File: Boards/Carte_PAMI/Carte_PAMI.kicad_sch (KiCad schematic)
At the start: 41 parts, among them J1 Emergency BTN, J10 DC Motor B, J2 USB_C_Receptacle_USB2.0_16P, J3 VL53L0X_1, J4 VL53L0X_2, J5 Battery_connector, J6 ELRS_Module, J7 Tirette, J8 DC Motor A, J9 Odom_Shield, Q1 PMOS, SW1 SW_Push, SW2 SW_Push, SW3 SW_Nidec_CAS-120A1, U1 ESP32-S3-WROOM-1U-N16R8, U2 USBLC6-2SC6, U3 TLV76150DCY, U4 TLV76133DCY, U5 TB6612FNG

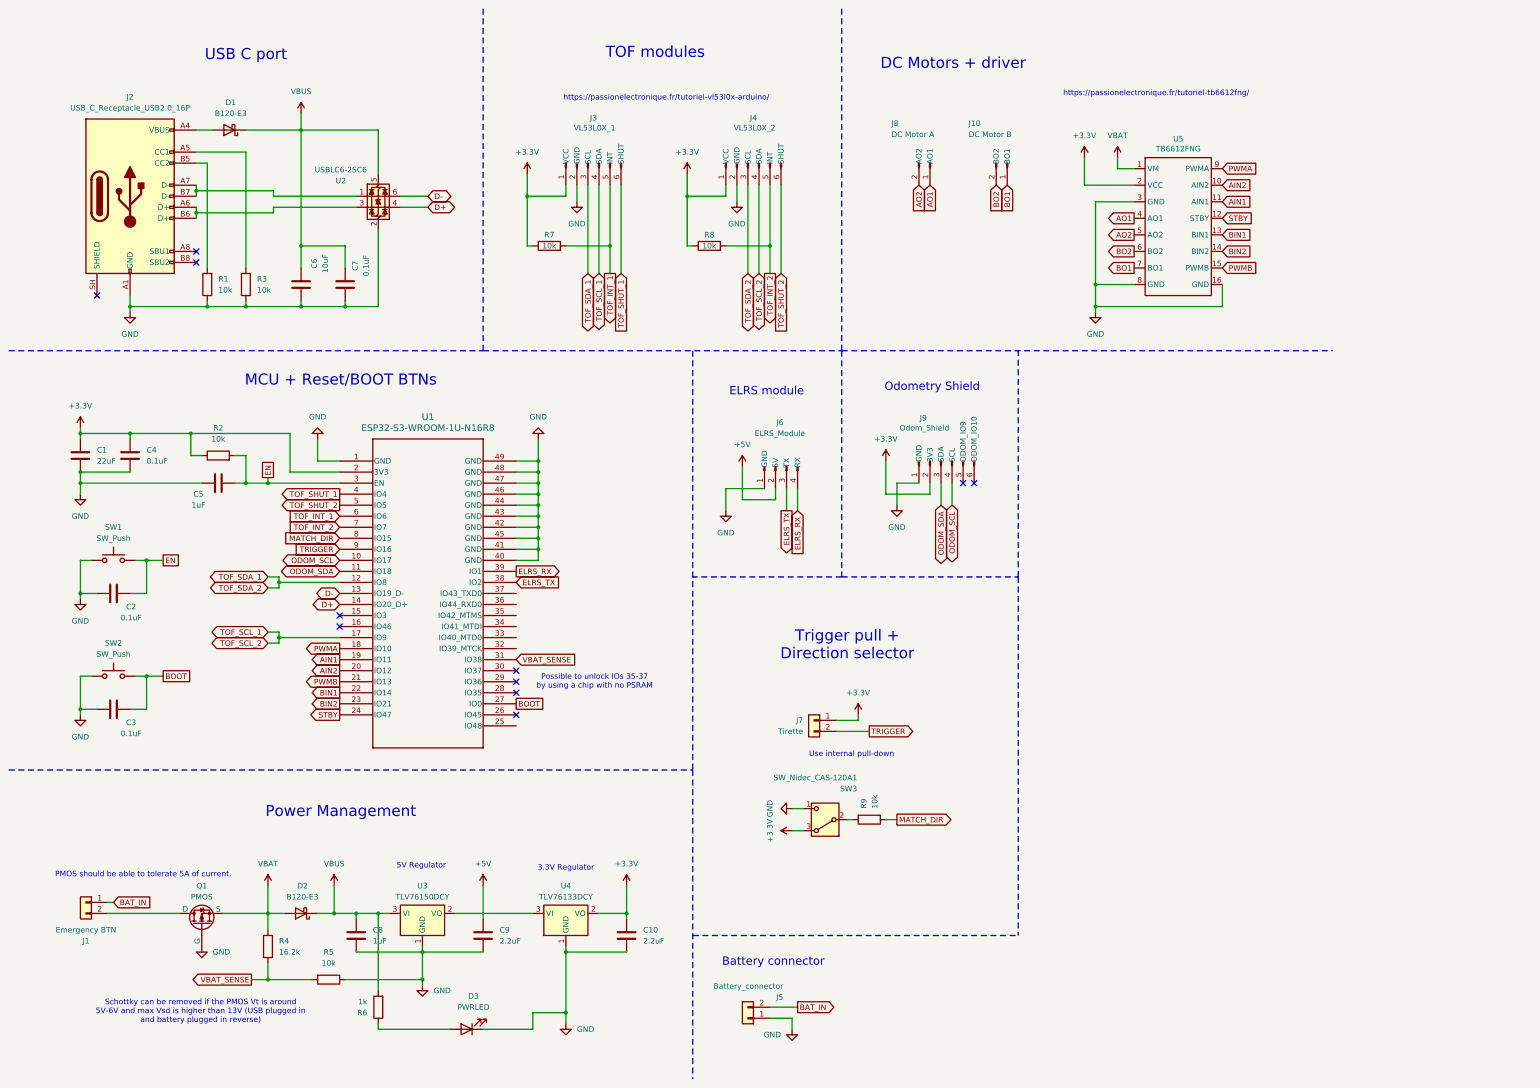
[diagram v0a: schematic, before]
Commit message: V1.1 : first layout
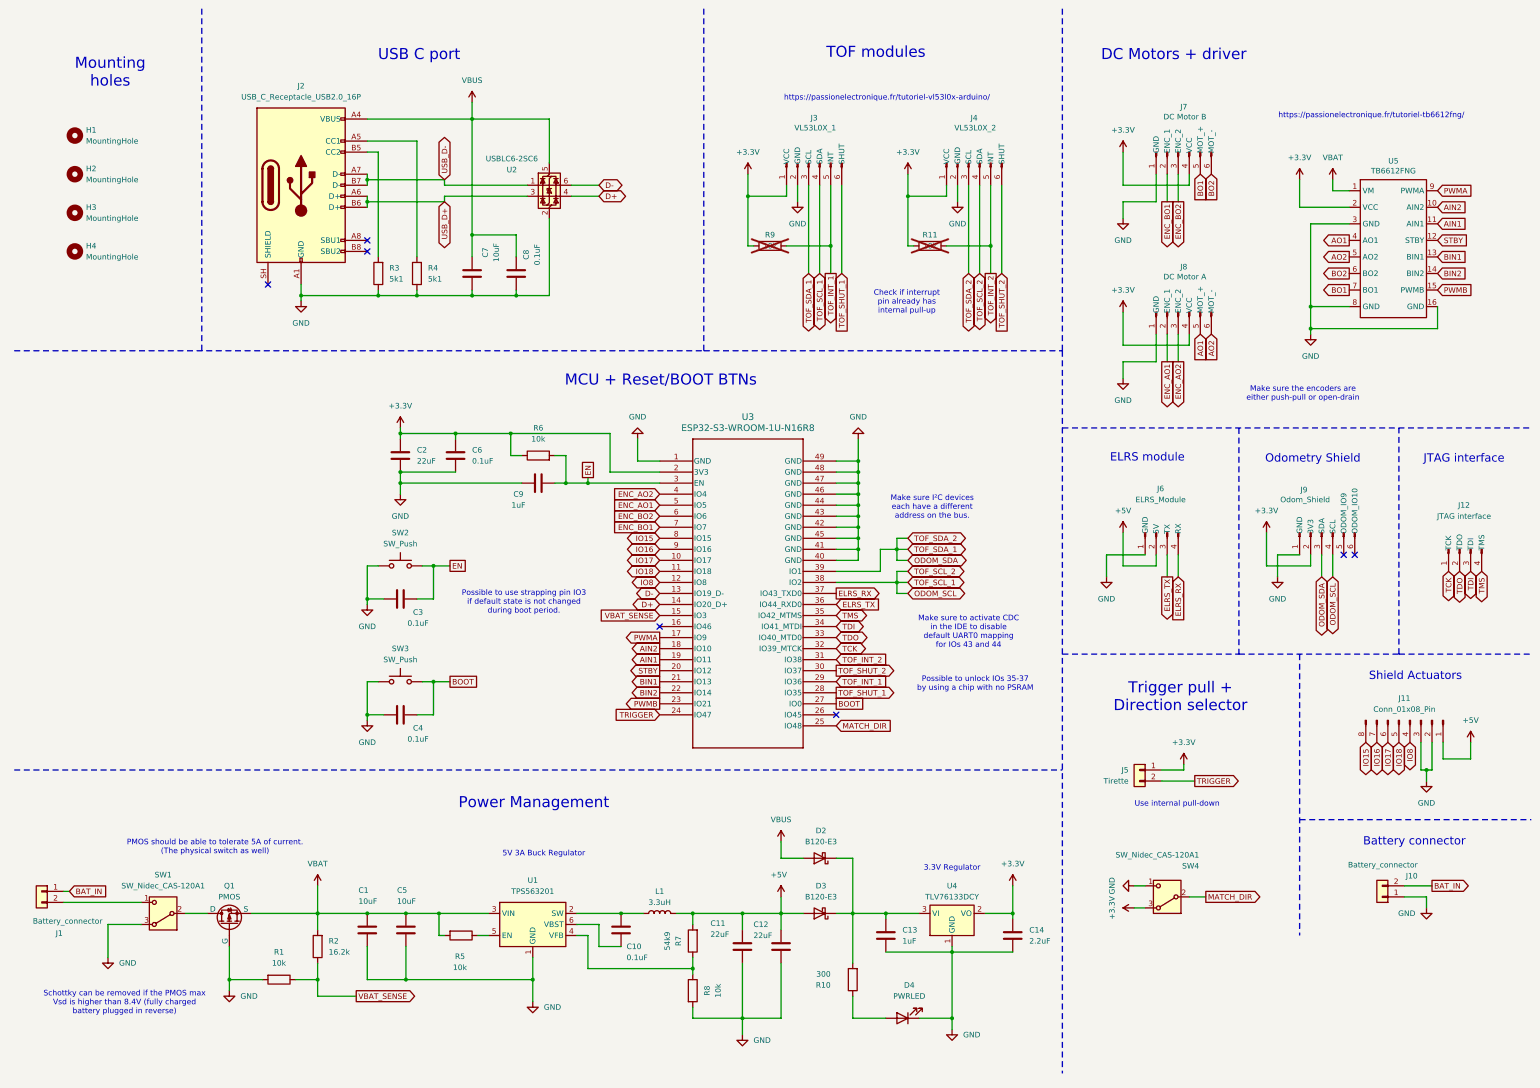
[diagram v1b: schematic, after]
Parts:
- removed C8: 1uF, Capacitor_SMD:C_0805_2012Metric, symbol Device:C
- removed C9: 2.2uF, Capacitor_SMD:C_0805_2012Metric, symbol Device:C
- removed J10: DC Motor B, Connector_PinHeader_2.54mm:PinHeader_1x02_P2.54mm_Vertical, symbol Connector:Conn_01x02_Pin
- removed J8: DC Motor A, Connector_PinHeader_2.54mm:PinHeader_1x02_P2.54mm_Vertical, symbol Connector:Conn_01x02_Pin
- removed R9: 10k, Resistor_SMD:R_1206_3216Metric, symbol Device:R
- removed U3: TLV76150DCY, Package_TO_SOT_SMD:SOT-223-3_TabPin2, symbol Regulator_Linear:TLV76150DCY
- added C1, C5: 10uF, Capacitor_SMD:C_0805_2012Metric, symbol Device:C
- added C10: 0.1uF, Capacitor_SMD:C_0805_2012Metric, symbol Device:C
- added C11, C12: 22uF, Capacitor_SMD:C_0805_2012Metric, symbol Device:C
- added C13: 1uF, Capacitor_SMD:C_0805_2012Metric, symbol Device:C
- added H1, H2, H3, H4: MountingHole, MountingHole:MountingHole_2.2mm_M2, symbol Mechanical:MountingHole
- added J11: Conn_01x08_Pin, Connector_PinHeader_2.54mm:PinHeader_1x08_P2.54mm_Vertical, symbol Connector:Conn_01x08_Pin
- added J12: JTAG interface, Connector_PinHeader_2.54mm:PinHeader_1x04_P2.54mm_Vertical, symbol Connector:Conn_01x04_Pin
- added J7: DC Motor B, Connector_PinHeader_2.54mm:PinHeader_1x06_P2.54mm_Vertical, symbol Connector:Conn_01x06_Pin
- added J8: DC Motor A, Connector_PinHeader_2.54mm:PinHeader_1x06_P2.54mm_Vertical, symbol Connector:Conn_01x06_Pin
- added L1: 3.3uH, Inductor_SMD:L_0805_2012Metric, symbol Device:L
- added R5, R8: 10k, Resistor_SMD:R_1206_3216Metric, symbol Device:R
- added R7: 54k9, Resistor_SMD:R_1206_3216Metric, symbol Device:R
- added SW1: SW_Nidec_CAS-120A1, Button_Switch_SMD:Nidec_Copal_CAS-120A, symbol Switch:SW_Nidec_CAS-120A1
- added U1: TPS563201, Package_TO_SOT_SMD:SOT-23-6, symbol Regulator_Switching:TPS563201
- J1: value Emergency BTN -> Battery_connector
- R10: renamed from R6; value 1k -> 300
- R11: renamed from R8; now not fitted; now left out of the parts list
- R3: renamed from R1; value 10k -> 5k1
- R4: renamed from R3; value 10k -> 5k1
- R9: renamed from R7; now not fitted; now left out of the parts list
- renumbered C10 to C14, C1 to C2, C2 to C3, C3 to C4, C4 to C6, C6 to C7, C7 to C8, C5 to C9, D1 to D3, D3 to D4, J5 to J10, J7 to J5, R5 to R1, R4 to R2, R2 to R6, SW1 to SW2, SW2 to SW3, SW3 to SW4, U1 to U3
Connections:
- net +3.3V: now also J7.4 (VCC), J8.4 (VCC)
- net +5V: now also D3.2 (A), C11.1, C12.1, J11.1 (Pin_1), L1.2, R7.2
- net AIN2: now also U3.18 (IO10); no longer U3.20 (IO12)
- net AO1: now also J8.5 (MOT_+)
- net AO2: now also J8.6 (MOT_-)
- net BIN1: now also U3.21 (IO13); no longer U3.22 (IO14)
- net BIN2: now also U3.22 (IO14); no longer U3.23 (IO21)
- net BO1: now also J7.5 (MOT_+)
- net BO2: now also J7.6 (MOT_-)
- net ELRS_RX: now also U3.37 (IO43_TXD0); no longer U3.39 (IO1)
- net ELRS_TX: now also U3.36 (IO44_RXD0); no longer U3.38 (IO2)
- net GND: now also R1.2, C1.2, C11.2, C12.2, C13.2, C5.2, J11.2 (Pin_2), J11.3 (Pin_3), J7.1 (GND), J8.1 (GND), R8.2, SW1.3 (A), U1.1 (GND); no longer R1.1
- net MATCH_DIR: now also SW4.2 (B), U3.25 (IO48); no longer U3.8 (IO15)
- net ODOM_SCL: now also J3.4 (SDA), J4.4 (SDA), U3.38 (IO2); no longer U3.10 (IO17)
- net ODOM_SDA: now also J3.3 (SCL), J4.3 (SCL), U3.39 (IO1); no longer U3.11 (IO18)
- net PWMA: now also U3.17 (IO9); no longer U3.18 (IO10)
- net PWMB: now also U3.23 (IO21); no longer U3.21 (IO13)
- net STBY: now also U3.20 (IO12); no longer U3.24 (IO47)
- net TOF_INT_1: now also U3.29 (IO36); no longer U3.6 (IO6)
- net TOF_INT_2: now also U3.31 (IO38); no longer U3.7 (IO7)
- net TOF_SHUT_1: now also U3.28 (IO35); no longer U3.4 (IO4)
- net TOF_SHUT_2: now also U3.30 (IO37); no longer U3.5 (IO5)
- net TRIGGER: now also U3.24 (IO47); no longer U3.9 (IO16)
- net VBAT: now also C1.1, C5.1, R5.2, U1.3 (VIN); no longer D2.2 (A)
- net VBAT_SENSE: now also R1.1, U3.15 (IO3); no longer R1.2, U3.31 (IO38)
- net VBUS: now also D2.2 (A), J2.A4 (VBUS), J2.A9 (VBUS), J2.B4 (VBUS), J2.B9 (VBUS); no longer D2.1 (K), D3.1 (K), R10.2
- net TCK: now reaches U3.32 (IO39_MTCK)
- net TCK: now also J12.1 (TCK)
- net TDO: now reaches U3.33 (IO40_MTD0)
- net TDO: now also J12.2 (TDO)
- net TDI: now reaches U3.34 (IO41_MTDI)
- net TDI: now also J12.3 (TDI)
- net TMS: now reaches U3.35 (IO42_MTMS)
- net TMS: now also J12.4 (TMS)
- net USB_D+: now reaches J2.A6 (D+), J2.B6 (D+), U2.3 (I/O2)
- net USB_D-: now reaches J2.A7 (D-), J2.B7 (D-), U2.1 (I/O1)
- net at U4.3 (VI): now also D2.1 (K), D3.1 (K), R10.2, C13.1
- net at Q1.1 (D): now also SW1.2 (B); no longer J1.2 (Pin_2)
- removed net TOF_SCL_1: J3.4 (SDA), J4.4 (SDA), U3.17 (IO9)
- removed net TOF_SDA_1: J3.3 (SCL), J4.3 (SCL), U3.12 (IO8)
- new net: C10.1, L1.1, U1.2 (SW)
- new net: R7.1, R8.1, U1.4 (VFB)
- new net: R5.1, U1.5 (EN)
- new net: C10.2, U1.6 (VBST)
- new net: J1.2 (Pin_2), SW1.1 (C)
- new net ENC_AO1: J8.2 (ENC_1), U3.5 (IO5)
- new net ENC_AO2: J8.3 (ENC_2), U3.4 (IO4)
- new net ENC_BO1: J7.2 (ENC_1), U3.7 (IO7)
- new net ENC_BO2: J7.3 (ENC_2), U3.6 (IO6)
- new net IO15: J11.8 (Pin_8), U3.8 (IO15)
- new net IO16: J11.7 (Pin_7), U3.9 (IO16)
- new net IO17: J11.6 (Pin_6), U3.10 (IO17)
- new net IO18: J11.5 (Pin_5), U3.11 (IO18)
- new net IO8: J11.4 (Pin_4), U3.12 (IO8)
- no-connect marks 11 -> 7
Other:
- note added: "5V 3A Buck Regulator"
- note added: "Check if interrupt pin already has internal pull-up"
- note added: "JTAG interface"
- note added: "Make sure I²C devices each have a different address on the bus."
- note added: "Make sure the encoders are either push-pull or open-drain"
- note added: "Make sure to activate CDC in the IDE to disable default UART0 mapping for IOs 43 and 44"
- note added: "Mounting holes"
- note added: "PMOS should be able to tolerate 5A of current. (The physical switch as well)"
- note added: "Possible to use strapping pin IO3 if default state is not changed during boot period."
- note added: "Schottky can be removed if the PMOS max Vsd is higher than 8.4V (fully charged battery plugged in reverse)"
- note added: "Shield Actuators"
- note removed: "5V Regulator"
- note removed: "PMOS should be able to tolerate 5A of current."
- note removed: "Schottky can be removed if the PMOS Vt is around 5V-6V and max Vsd is higher than 13V (USB plugged in and battery plugged in reverse)"
- moved on the sheet: C14, C2, C3, C4, C6, C7, C8, C9, D3, D4, J10, J2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
